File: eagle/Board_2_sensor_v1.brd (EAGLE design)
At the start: 14 x 57 mm, 20 parts, among them CN2 M02JST-PTH-2, IC7 TLV71333DBV, U1 MCP3421, U2 MCP73831, X1 Micro USB

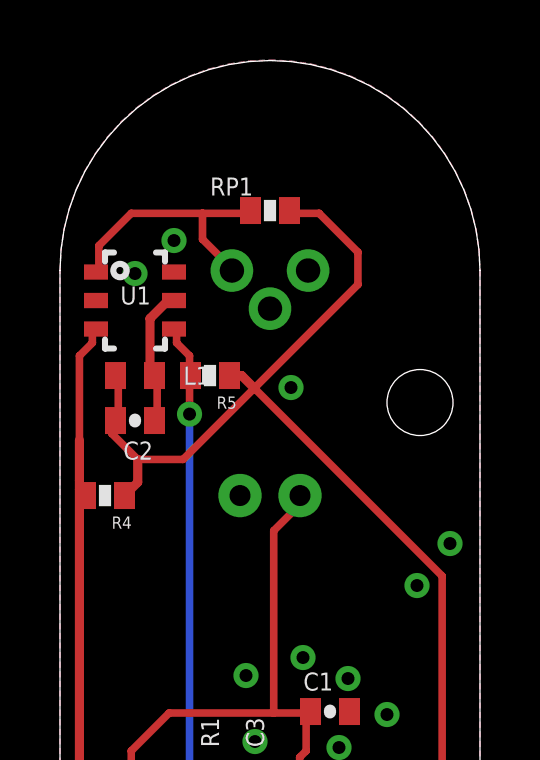
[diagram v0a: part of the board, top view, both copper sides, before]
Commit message: Latest Update, research files added
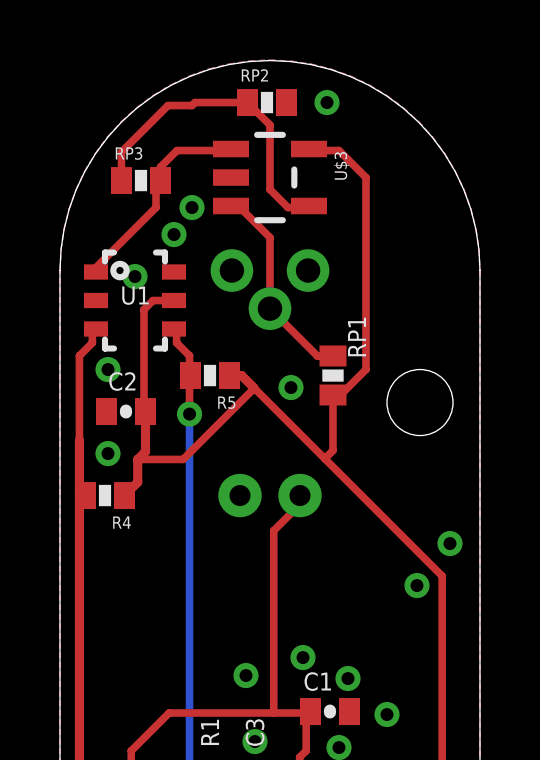
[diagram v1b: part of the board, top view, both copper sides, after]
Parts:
- removed L1: (no value), SparkFun-Passives:C0402
- added RP2: 22k, SparkFun:0402-RES
- added RP3: 180k, SparkFun:0402-RES
- added U$3: OPA344, SparkFun-AnalogIC:SOT23-5
- moved RP1 5.89 mm to (9.10, 39.5), turned to 90 degrees
- moved C2 0.42 mm to (2.20, 38.3), turned to 180 degrees
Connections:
- removed net N$1: C2.2, L1.2, U1.5
- removed net N$5: LED1.C, RP1.2, U1.1
- new net N$2: LED1.A, RP1.2, U$3.3
- new net N$3: RP2.1, RP3.1, U$3.4
- new net N$4: RP3.2, U$3.1, U1.1
- net GND: now also C2.2, LED1.C, RP2.2, U$3.2; no longer LED1.A
- net VCC: now also U$3.5, U1.5; no longer L1.1
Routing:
- net N$3: track 0.00 -> 10.6 mm
- net N$5: track 8.80 -> 0.00 mm
- net N$4: track 0.00 -> 6.99 mm
- net N$2: track 0.00 -> 6.86 mm
- net VCC: track 66.1 -> 72.6 mm
- net N$1: track 4.55 -> 0.00 mm
